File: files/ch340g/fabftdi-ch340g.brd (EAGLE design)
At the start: 58.1 x 28.1 mm, 12 parts, among them U1 CH340G, Y1 12MHz

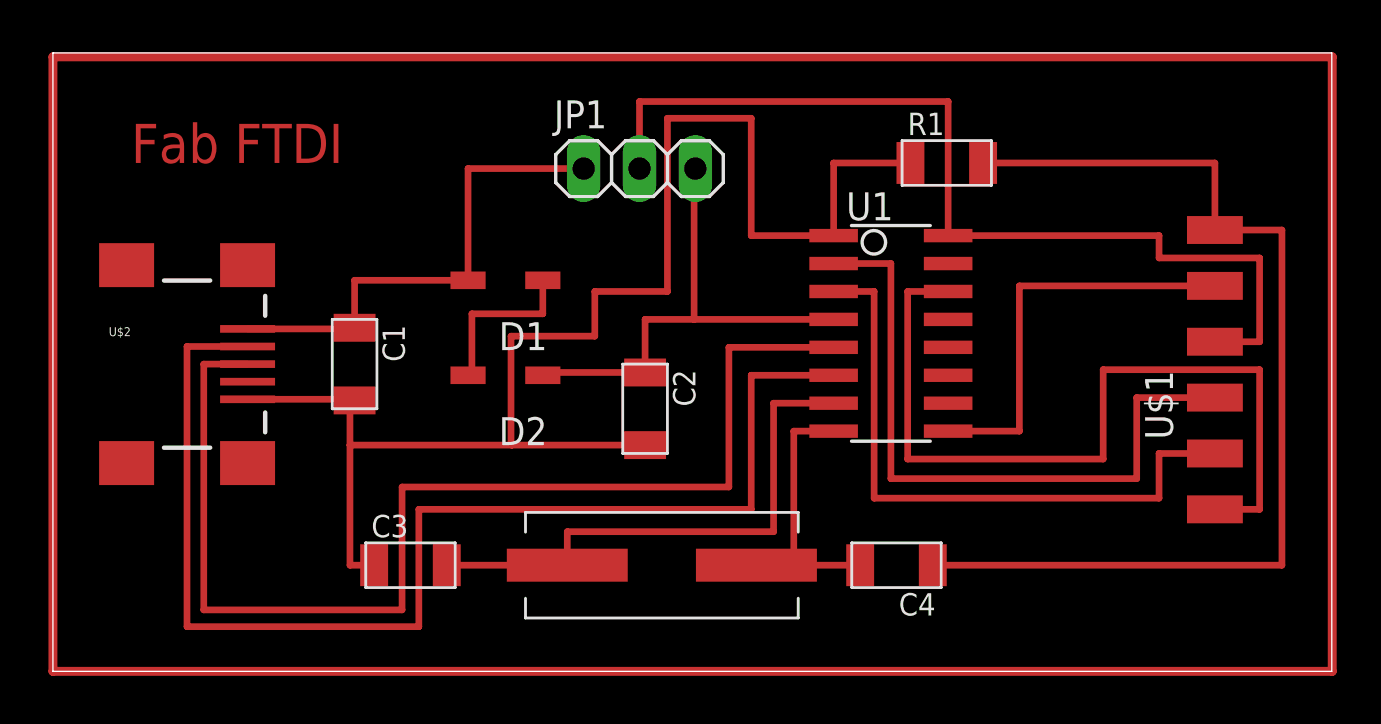
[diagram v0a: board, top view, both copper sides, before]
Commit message: updated all files, added components list
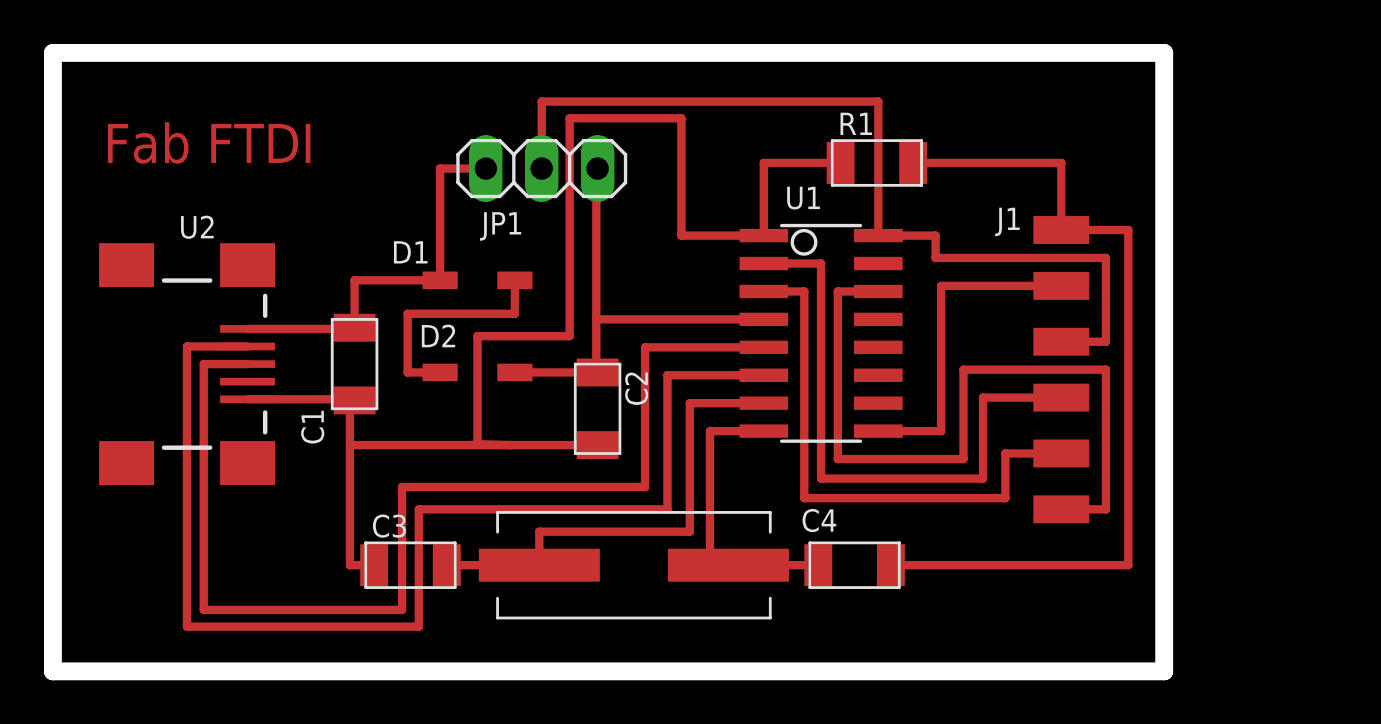
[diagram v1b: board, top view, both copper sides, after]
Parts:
- removed U$1: FTDI-SMD-HEADER, 00fab:1X06SMD
- added J1: FTDI, 00fab:1X06SMD
- moved JP1 4.45 mm to (22.2, 22.9)
- moved U1 3.18 mm to (34.9, 16.0)
- moved R1 3.17 mm to (37.5, 23.1)
- moved C2 2.16 mm to (24.8, 11.9)
- moved C4 1.91 mm to (36.4, 4.83)
- moved D2 1.28 mm to (19.3, 13.6)
- moved D1 1.27 mm to (19.3, 17.8)
- moved Y1 1.27 mm to (26.4, 4.83)
- renumbered U$2 to U2
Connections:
- net GND': now also J1.1; no longer U$1.1
- net N$10: now also J1.4; no longer U$1.4
- net N$11: now also J1.5; no longer U$1.5
- net N$12: now also J1.6; no longer U$1.6
- net N$9: now also J1.2; no longer U$1.2
- net VCC: now also J1.3; no longer U$1.3
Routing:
- net N$3: track 172.2 -> 157.0 mm
- net GND': track 47.8 -> 38.9 mm
- net 5V: track 22.6 -> 18.1 mm
- net N$9: track 19.2 -> 15.4 mm
- net N$11: track 28.8 -> 25.0 mm
- net N$10: track 30.8 -> 27.0 mm
- net N$12: track 37.9 -> 34.1 mm
- net N$2: track 25.0 -> 21.8 mm
- net D-: track 56.3 -> 53.1 mm
- net D+: track 53.7 -> 50.6 mm
- net N$4: track 7.72 -> 10.5 mm
- net VCC: track 44.2 -> 41.7 mm
- net GND: track 68.6 -> 66.3 mm
- net 3V3: track 22.7 -> 20.7 mm
- net N$1: track 12.6 -> 13.5 mm
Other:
- board size 58.1 x 28.1 mm -> 50.5 x 28.1 mm
- board text added: "12 MHz"
- board text added: "3V"
- board text added: "5V"
